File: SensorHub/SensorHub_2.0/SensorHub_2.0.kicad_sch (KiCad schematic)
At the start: 9 parts, among them J1 USB_B_Micro, U1 R7FA4E2B93CFM#AA0, U2 AP2112K-3.3

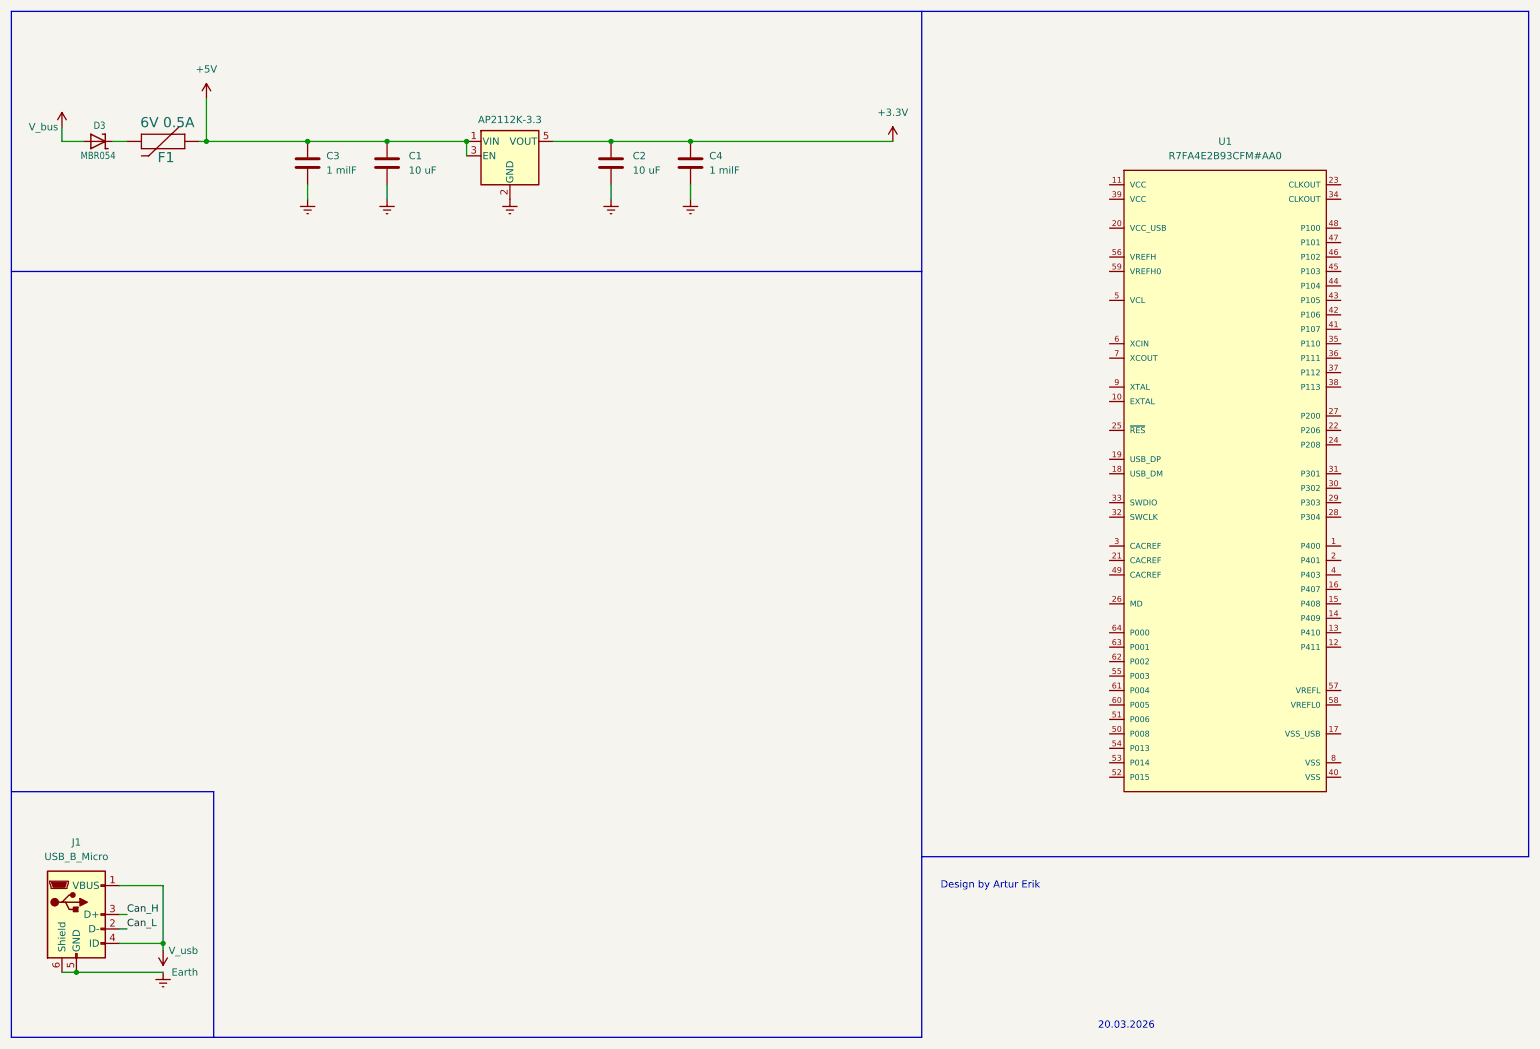
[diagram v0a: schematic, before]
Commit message: 1st version SensorHub
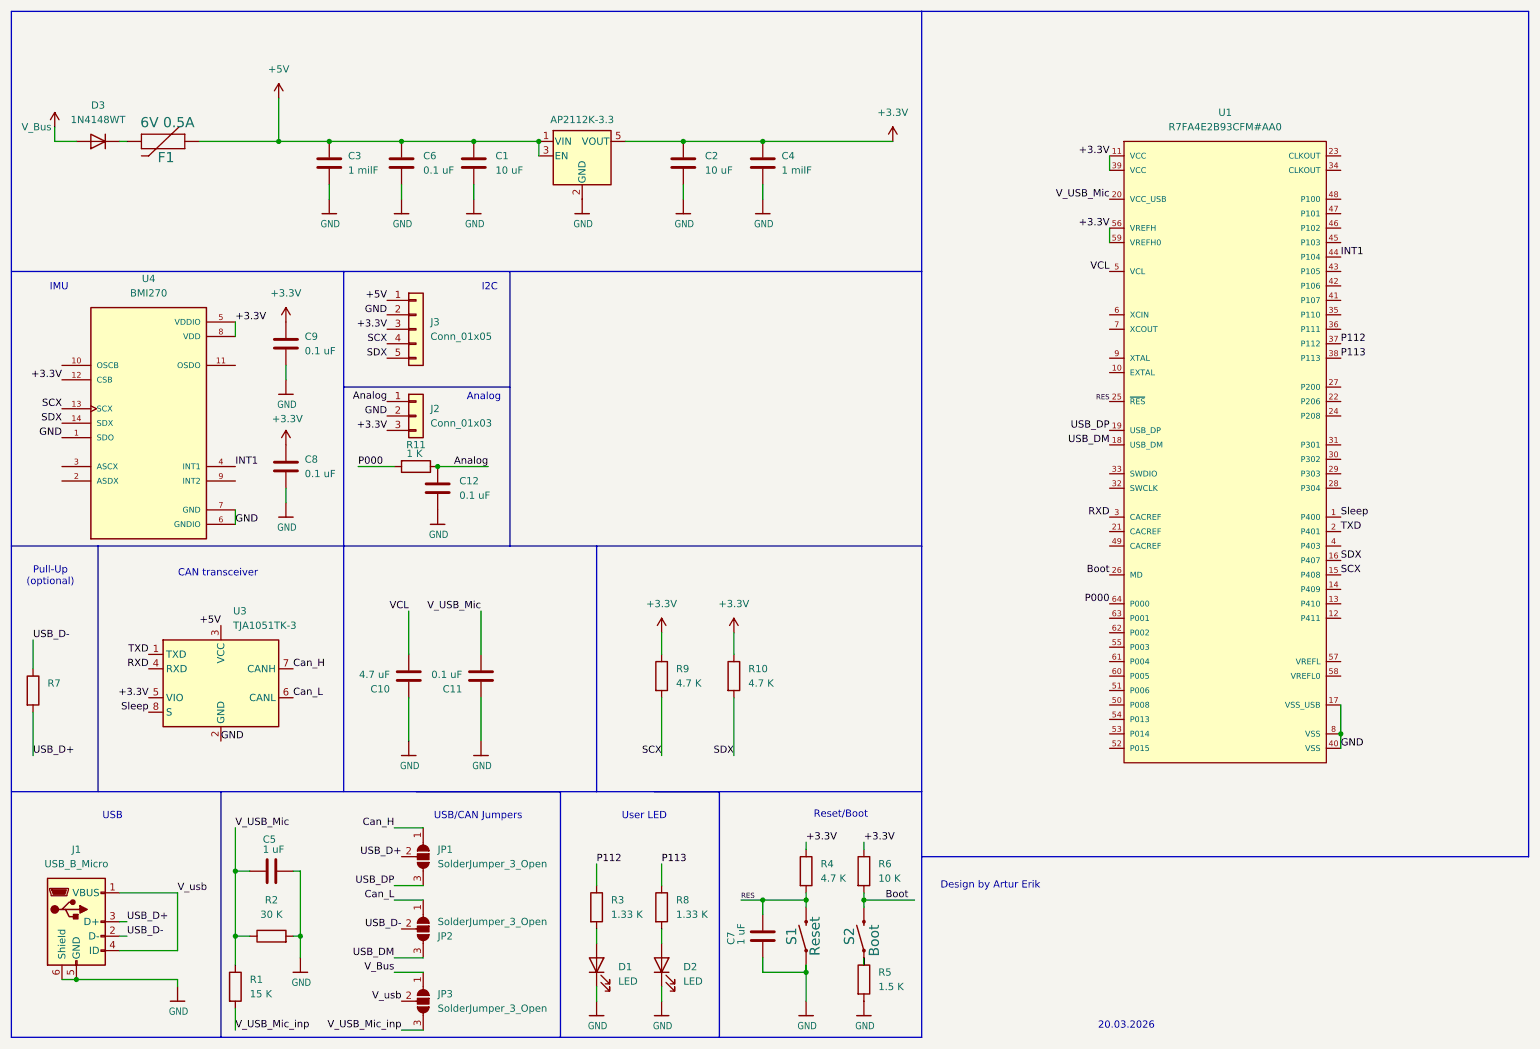
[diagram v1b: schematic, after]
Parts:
- removed D3: MBR054, SensorHub MicroMod Carrier v1.1.0b:SOD-123, symbol SensorHub MicroMod Carrier v1.1.0b-eagle-import:DIODE-SCHOTTKYSOD-123
- added C10: 4.7 uF, Capacitor_SMD:C_0603_1608Metric, symbol Device:C
- added C11, C12, C6, C8, C9: 0.1 uF, Capacitor_SMD:C_0603_1608Metric, symbol Device:C
- added C5, C7: 1 uF, Capacitor_SMD:C_0603_1608Metric, symbol Device:C
- added D1, D2: LED, LED_SMD:LED_0402_1005Metric, symbol Device:LED
- added D3: 1N4148WT, Diode_SMD:D_SOD-523, symbol Diode:1N4148WT
- added J2: Conn_01x03, Connector_PinHeader_2.54mm:PinHeader_1x03_P2.54mm_Vertical, symbol Connector_Generic:Conn_01x03
- added J3: Conn_01x05, Connector_PinHeader_2.54mm:PinHeader_1x05_P2.54mm_Vertical, symbol Connector_Generic:Conn_01x05
- added JP1, JP2, JP3: SolderJumper_3_Open, Jumper:SolderJumper-3_P1.3mm_Open_RoundedPad1.0x1.5mm, symbol Jumper:SolderJumper_3_Open
- added R1: 15 K, Resistor_SMD:R_0201_0603Metric, symbol Device:R
- added R10, R4, R9: 4.7 K, Resistor_SMD:R_0201_0603Metric, symbol Device:R
- added R11: 1 K, Resistor_SMD:R_0201_0603Metric, symbol Device:R
- added R2: 30 K, Resistor_SMD:R_0201_0603Metric, symbol Device:R
- added R3, R8: 1.33 K, Resistor_SMD:R_0201_0603Metric, symbol Device:R
- added R5: 1.5 K, Resistor_SMD:R_0201_0603Metric, symbol Device:R
- added R6: 10 K, Resistor_SMD:R_0201_0603Metric, symbol Device:R
- added R7: ~, Resistor_SMD:R_0201_0603Metric, symbol Device:R
- added S1: Reset, Library:Button_Mini_2.5x1.7mm, symbol SensorHub MicroMod Carrier v1.1.0b-eagle-import:MOMENTARY-SWITCH-SPST-SMD-5.2-T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
- added S2: Boot, Library:Button_Mini_2.5x1.7mm, symbol SensorHub MicroMod Carrier v1.1.0b-eagle-import:MOMENTARY-SWITCH-SPST-SMD-5.2-T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
- added U3: TJA1051TK-3, Package_SON:HVSON-8-1EP_3x3mm_P0.65mm_EP1.6x2.4mm, symbol Interface_CAN_LIN:TJA1051TK-3
- added U4: BMI270, BMI270:XDCR_BMI270, symbol BMI270:BMI270
- C1, C2, C3, C4: footprint (none) -> Capacitor_SMD:C_0603_1608Metric
- J1: footprint (none) -> Connector_USB:USB_Micro-B_Molex-105017-0001
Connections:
- net Earth is gone; now on net GND: C1.2, C2.2, C3.2, C4.2, J1.5 (GND), J1.6 (Shield), U2.2 (GND)
- net +3.3V: now also U1.11 (VCC), U1.39 (VCC), U1.56 (VREFH), U1.59 (VREFH0), C8.1, C9.1, J2.3 (Pin_3), J3.3 (Pin_3), R10.1, R4.1, R6.1, R9.1, U3.5 (VIO), U4.12 (CSB), U4.5 (VDDIO), U4.8 (VDD)
- net +5V: now also C6.1, J3.1 (Pin_1), U3.3 (VCC)
- net Can_H: now also JP1.1 (A), U3.7 (CANH); no longer J1.3 (D+)
- net Can_L: now also JP2.1 (A), U3.6 (CANL); no longer J1.2 (D-)
- net V_usb: now also JP3.2 (C)
- net Sleep: now reaches U1.1 (P400)
- net Sleep: now also U3.8 (S)
- net SCX: now reaches U1.15 (P408)
- net SCX: now also J3.4 (Pin_4), R9.2, U4.13 (SCX)
- net SDX: now reaches U1.16 (P407)
- net SDX: now also J3.5 (Pin_5), R10.2, U4.14 (SDX)
- net GND: now reaches U1.17 (VSS_USB)
- net GND: now also U1.40 (VSS), U1.8 (VSS), C10.2, C11.2, C12.2, C5.1, C6.2, C7.2, C8.2, C9.2, D1.1 (K), D2.1 (K), J2.2 (Pin_2), J3.2 (Pin_2), R2.2, R5.2, S1.1, S1.2 (1), U3.2 (GND), U3.9 (GND), U4.1 (SDO), U4.6 (GNDIO), U4.7 (GND)
- net USB_DM: now reaches U1.18 (USB_DM)
- net USB_DM: now also JP2.3 (B)
- net USB_DP: now reaches U1.19 (USB_DP)
- net USB_DP: now also JP1.3 (B)
- net TXD: now reaches U1.2 (P401)
- net TXD: now also U3.1 (TXD)
- net V_USB_Mic: now reaches U1.20 (VCC_USB)
- net V_USB_Mic: now also C11.1, C5.2, R1.1, R2.1
- net RES: now reaches U1.25 (~{RES})
- net RES: now also C7.1, R4.2, S1.3 (2), S1.4 (2)
- net Boot: now reaches U1.26 (MD)
- net Boot: now also R6.2, S2.3 (2), S2.4 (2)
- net RXD: now reaches U1.3 (CACREF)
- net RXD: now also U3.4 (RXD)
- net P112: now reaches U1.37 (P112)
- net P112: now also R3.1
- net P113: now reaches U1.38 (P113)
- net P113: now also R8.1
- net INT1: now reaches U1.44 (P104)
- net INT1: now also U4.4 (INT1)
- net VCL: now reaches U1.5 (VCL)
- net VCL: now also C10.1
- net P000: now reaches U1.64 (P000)
- net P000: now also R11.2
- net at F1.2: now also D3.1 (K)
- new net: R5.1, S2.1, S2.2 (1)
- new net: D2.2 (A), R8.2
- new net: D1.2 (A), R3.2
- new net Analog: C12.1, J2.1 (Pin_1), R11.1
- new net USB_D+: J1.3 (D+), JP1.2 (C), R7.2
- new net USB_D-: J1.2 (D-), JP2.2 (C), R7.1
- new net V_Bus: D3.2 (A), JP3.1 (A)
- new net V_USB_Mic_inp: JP3.3 (B), R1.2
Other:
- note added: "Analog"
- note added: "CAN transceiver"
- note added: "I2C"
- note added: "IMU"
- note added: "Pull-Up (optional)"
- note added: "Reset/Boot"
- note added: "USB"
- note added: "USB/CAN Jumpers"
- note added: "User LED"
- moved on the sheet: C1, C2, C3, C4, J1, U1
